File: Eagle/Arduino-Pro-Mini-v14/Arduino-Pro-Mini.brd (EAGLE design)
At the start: 30 x 32.8 mm, 26 parts, among them J1 BM04B-GHS-TBT(LF)(SN)(N), J2 SM08B-GHS-TB(LF)(SN), J3 SM08B-GHS-TB(LF)(SN), Q1 8/16/20MHz, Q2 BCW65CLT1G, Q3 BCW65CLT1G, Q4 BCW65CLT1G, U1 ATMEGA328, U2 MIC5205

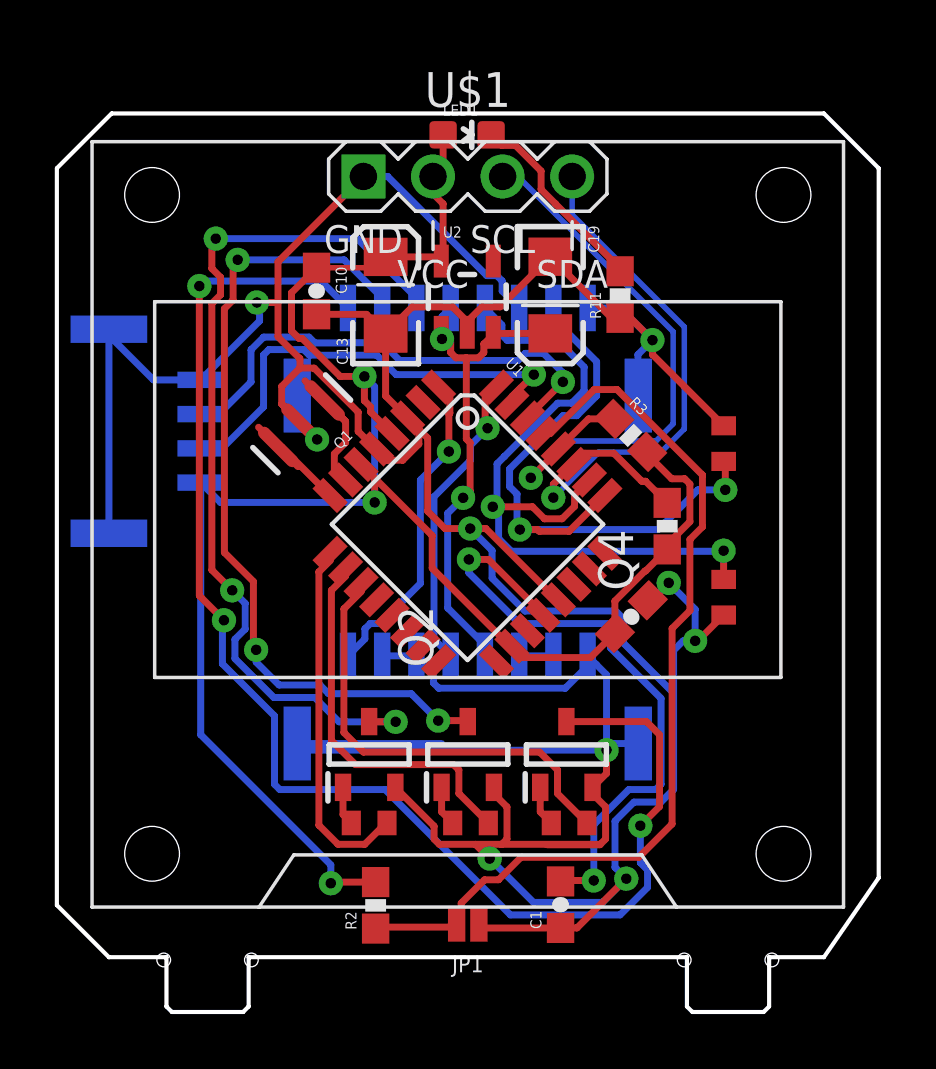
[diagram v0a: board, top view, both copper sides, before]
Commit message: LED board
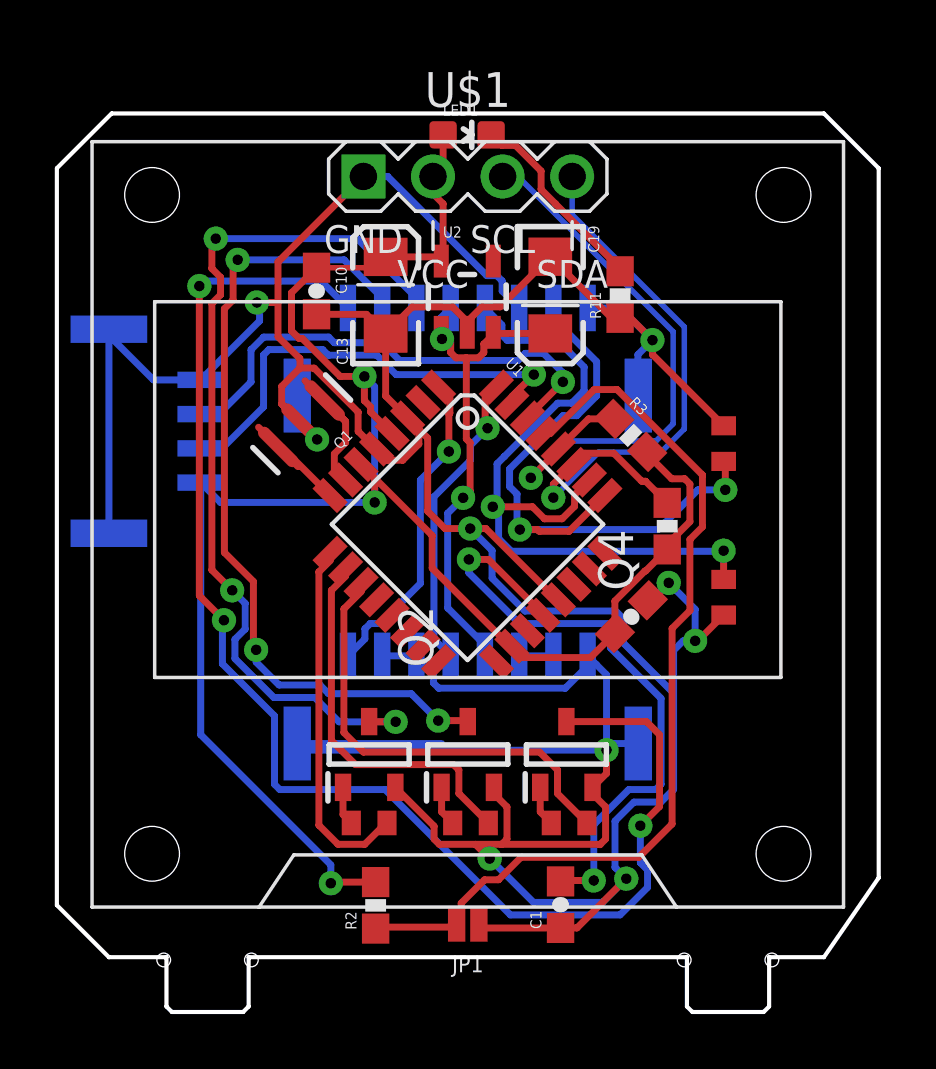
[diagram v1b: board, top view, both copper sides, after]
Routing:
- net GND: track 171.4 -> 169.5 mm
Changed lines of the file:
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@@
 <drawing>
 <settings>
-<setting alwaysvectorfont="yes"/>
+<setting alwaysvectorfont="no"/>
 <setting keepoldvectorfont="yes"/>
 <setting verticaltext="up"/>
@@
 <wire x1="20.0302" y1="3.513225" x2="19.836775" y2="3.3198" width="0.254" layer="1"/>
 <wire x1="19.836775" y1="3.3198" x2="19.821784375" y2="3.304809375" width="0.254" layer="1"/>
-<wire x1="19.821784375" y1="3.304809375" x2="17.9" y2="3.304809375" width="0.254" layer="1"/>
 <wire x1="19.836775" y1="3.3198" x2="16.236775" y2="3.3198" width="0.254" layer="1"/>
 <wire x1="13.7448" y1="9.213225" x2="13.938225" y2="9.0198" width="0.254" layer="16"/>
@@
 <wire x1="17.411853125" y1="20.467453125" x2="16.6111125" y2="19.6667125" width="0.254" layer="1"/>
 <wire x1="16.6111125" y1="19.6667125" x2="16.6111125" y2="19.4495375" width="0.254" layer="1"/>
-<wire x1="11.67871875" y1="21.1747" x2="9.217275" y2="21.1747" width="0.254" layer="16"/>
+<wire x1="11.67871875" y1="21.1747" x2="9.907275" y2="21.1747" width="0.254" layer="16"/>
 <wire x1="6.033025" y1="17.775" x2="5.25" y2="17.775" width="0.254" layer="16"/>
 <wire x1="12.385965625" y1="20.467453125" x2="11.67871875" y2="21.1747" width="0.254" layer="16"/>
 <wire x1="17.411853125" y1="20.467453125" x2="12.385965625" y2="20.467453125" width="0.254" layer="16"/>
 <wire x1="7.5448" y1="19.286775" x2="6.033025" y2="17.775" width="0.254" layer="16"/>
-<wire x1="9.217275" y1="21.1747" x2="9.011775" y2="21.3802" width="0.254" layer="16"/>
-<wire x1="9.011775" y1="21.3802" x2="7.738225" y2="21.3802" width="0.254" layer="16"/>
+<wire x1="9.907275" y1="21.1747" x2="9.701775" y2="21.3802" width="0.254" layer="16"/>
+<wire x1="9.701775" y1="21.3802" x2="7.738225" y2="21.3802" width="0.254" layer="16"/>
 <wire x1="7.738225" y1="21.3802" x2="7.5448" y2="21.186775" width="0.254" layer="16"/>
 <wire x1="7.5448" y1="21.186775" x2="7.5448" y2="19.286775" width="0.254" layer="16"/>
@@
 <contactref element="U1" pad="30"/>
 <contactref element="J1" pad="2"/>
-<wire x1="7.54884375" y1="21.8374" x2="9.20115625" y2="21.8374" width="0.254" layer="16"/>
-<wire x1="10.70911875" y1="21.625" x2="10.71601875" y2="21.6319" width="0.254" layer="16"/>
-<wire x1="9.41355625" y1="21.625" x2="10.70911875" y2="21.625" width="0.254" layer="16"/>
-<wire x1="9.20115625" y1="21.8374" x2="9.41355625" y2="21.625" width="0.254" layer="16"/>
-<wire x1="10.71601875" y1="21.6319" x2="11.8681" y2="21.6319" width="0.254" layer="16"/>
+<wire x1="7.54884375" y1="21.8374" x2="9.92115625" y2="21.8374" width="0.254" layer="16"/>
+<wire x1="10.12665625" y1="21.6319" x2="11.8681" y2="21.6319" width="0.254" layer="16"/>
+<wire x1="9.92115625" y1="21.8374" x2="10.12665625" y2="21.6319" width="0.254" layer="16"/>
 <wire x1="12.517015625" y1="20.982984375" x2="11.8681" y2="21.6319" width="0.254" layer="16"/>
 <via x="18.4719125" y="20.2" extent="1-16" drill="0.381"/>
@@
 <wire x1="14.569025" y1="21.0797" x2="14.946" y2="21.0797" width="0.254" layer="1"/>
 <wire x1="15.392575" y1="21.0797" x2="15.586" y2="21.273125" width="0.254" layer="1"/>
-<wire x1="14.3756" y1="21.6651" x2="14.3756" y2="21.273125" width="0.254" layer="1"/>
+<wire x1="14.3756" y1="21.273125" x2="14.3756" y2="21.6651" width="0.254" layer="1"/>
 <wire x1="15.586" y1="21.273125" x2="15.586" y2="21.5853" width="0.254" layer="1"/>
 <wire x1="15.586" y1="21.5853" x2="15.9707" y2="21.97" width="0.254" layer="1"/>
-<wire x1="14.0308" y1="22.0099" x2="14.17035" y2="21.87035" width="0.254" layer="1"/>
 <contactref element="J2" pad="4"/>
 <via x="14.83" y="15.97" extent="1-16" drill="0.381"/>
-<wire x1="14.17035" y1="21.87035" x2="14.3756" y2="21.6651" width="0.254" layer="1"/>
 <wire x1="15.625" y1="10.59" x2="15.625" y2="10.2" width="0.254" layer="16"/>
 <wire x1="14.265" y1="11.95" x2="15.625" y2="10.59" width="0.254" layer="16"/>
@@
 <contactref element="J3" pad="5"/>
 <wire x1="14.946" y1="21.0797" x2="15.392575" y2="21.0797" width="0.254" layer="1"/>
-<wire x1="14.375" y1="22.9" x2="14.0581" y2="22.5831" width="0.254" layer="16"/>
-<wire x1="14.0581" y1="22.5831" x2="14.0581" y2="21.7671125" width="0.254" layer="16"/>
+<wire x1="13.9881" y1="22.5131" x2="14.375" y2="22.9" width="0.254" layer="16"/>
+<wire x1="14.3756" y1="21.6651" x2="14.0308" y2="22.0099" width="0.254" layer="1"/>
+<wire x1="14.0308" y1="22.0099" x2="14.0308" y2="21.7944125" width="0.254" layer="1"/>
+<wire x1="14.0308" y1="21.7944125" x2="14.0581" y2="21.7671125" width="0.254" layer="1"/>
 <via x="14.0581" y="21.7671125" extent="1-16" drill="0.381"/>
-<wire x1="14.0581" y1="21.7671125" x2="14.1613375" y2="21.87035" width="0.254" layer="1"/>
-<wire x1="14.1613375" y1="21.87035" x2="14.17035" y2="21.87035" width="0.254" layer="1"/>
+<wire x1="14.0581" y1="21.7671125" x2="13.9881" y2="21.8371125" width="0.254" layer="16"/>
+<wire x1="13.9881" y1="21.8371125" x2="13.9881" y2="22.5131" width="0.254" layer="16"/>
 </signal>
 <signal name="A2">
